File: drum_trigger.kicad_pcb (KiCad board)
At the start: 4 copper layers, 65 x 60 mm, 60 parts, among them J10 Conn_01x02_Pin, J11 Conn_01x02_Pin, J12 Conn_01x03_Pin, J4 Conn_01x03_Pin, J6 AudioJack2, J7 AudioJack2, U1 LM2902PWR

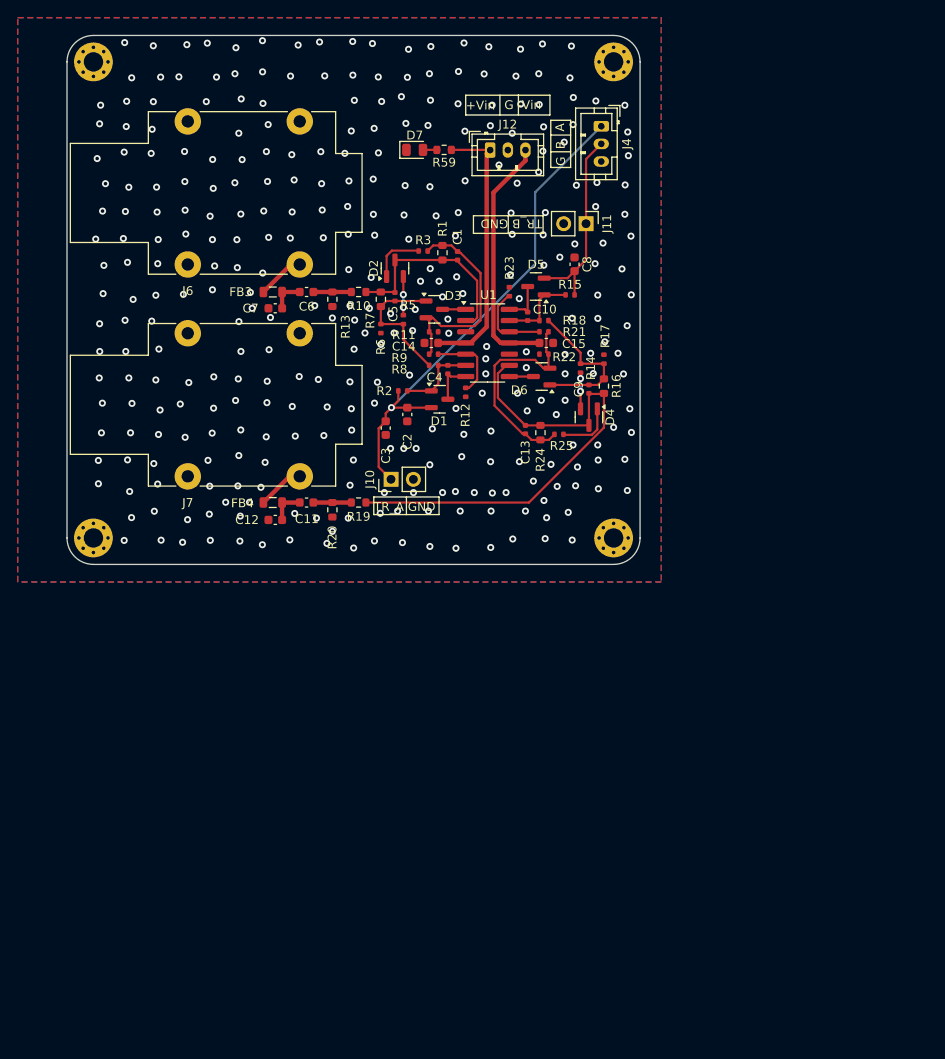
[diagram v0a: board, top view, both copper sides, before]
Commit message: Add channels
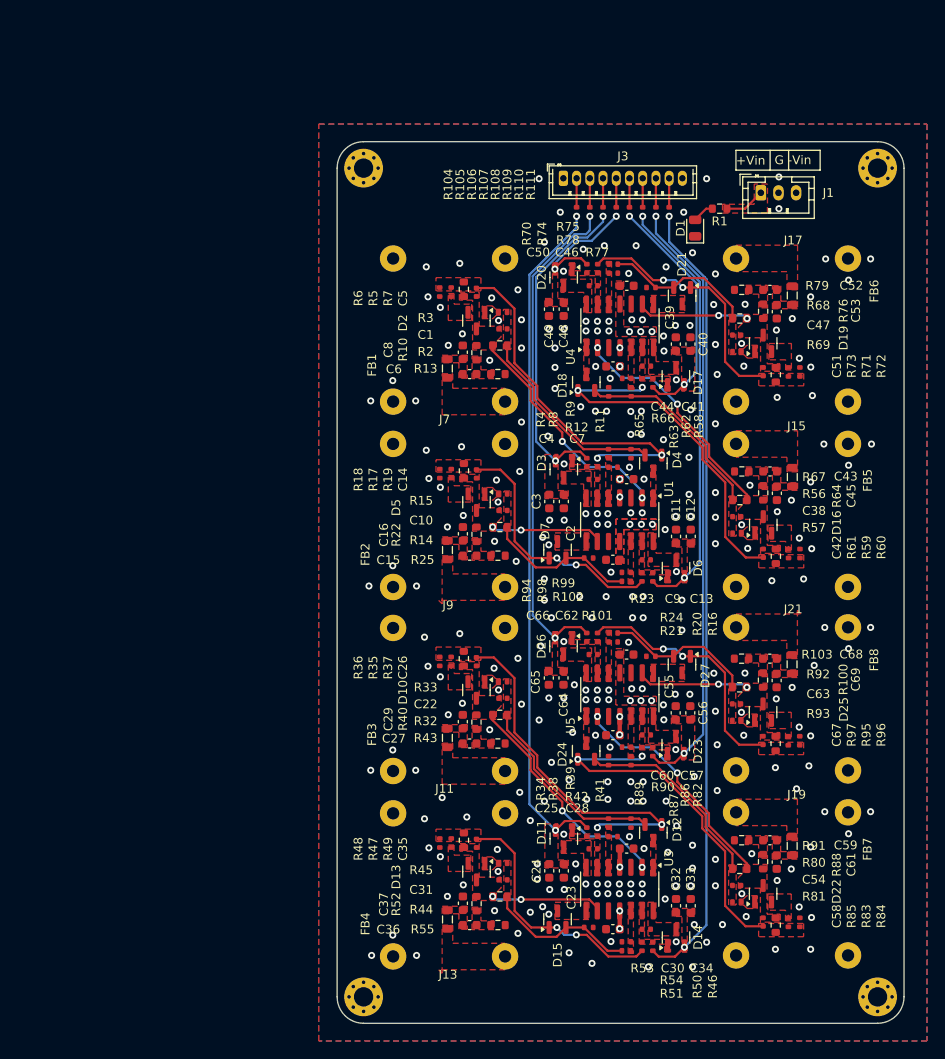
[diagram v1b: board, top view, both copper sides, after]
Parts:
- removed the D7 at (110.9, 42.9)
- removed J10: Conn_01x02_Pin, Connector_PinHeader_2.54mm:PinHeader_1x02_P2.54mm_Vertical
- removed J12, J4: Conn_01x03_Pin, Connector_JST:JST_PH_B3B-PH-K_1x03_P2.00mm_Vertical
- added C12: 1nF, Capacitor_SMD:C_0603_1608Metric, F.Cu at (142.2, 86.8)
- added C22: 22pF, C_0402_custom:C_0402_1005Metric, F.Cu at (120.9, 105.1)
- added C23: 220nF, Capacitor_SMD:C_0603_1608Metric, F.Cu at (127.8, 124.7)
- added C24: 1nF, Capacitor_SMD:C_0603_1608Metric, F.Cu at (126.2, 124.7)
- added C25: 22pF, C_0402_custom:C_0402_1005Metric, F.Cu at (131.1, 122.2)
- added C26: 22pF, C_0402_custom:C_0402_1005Metric, F.Cu at (117.9, 101.0)
- added C27: 220nF, Capacitor_SMD:C_0603_1608Metric, F.Cu at (117.1, 110.3)
- added C28: 1uF, Capacitor_SMD:C_0603_1608Metric, F.Cu at (134.9, 122.2)
- added C29: 100pF, Capacitor_SMD:C_0603_1608Metric, F.Cu at (116.4, 107.8)
- added C30: 1uF, Capacitor_SMD:C_0603_1608Metric, F.Cu at (133.4, 131.3)
- added C31: 22pF, C_0402_custom:C_0402_1005Metric, F.Cu at (120.9, 125.7)
- added C32: 220nF, Capacitor_SMD:C_0603_1608Metric, F.Cu at (140.5, 128.7)
- added C33: 1nF, Capacitor_SMD:C_0603_1608Metric, F.Cu at (142.2, 128.7)
- added C34: 22pF, C_0402_custom:C_0402_1005Metric, F.Cu at (137.2, 131.3)
- added C35: 22pF, C_0402_custom:C_0402_1005Metric, F.Cu at (117.9, 121.6)
- added C36: 220nF, Capacitor_SMD:C_0603_1608Metric, F.Cu at (117.1, 130.9)
- added C37: 100pF, Capacitor_SMD:C_0603_1608Metric, F.Cu at (116.4, 128.4)
- added C38: 22pF, C_0402_custom:C_0402_1005Metric, F.Cu at (147.4, 84.5)
- added C39: 220nF, Capacitor_SMD:C_0603_1608Metric, F.Cu at (140.5, 65.0)
- added C40: 1nF, Capacitor_SMD:C_0603_1608Metric, F.Cu at (142.2, 65.0)
- added C41: 22pF, C_0402_custom:C_0402_1005Metric, F.Cu at (137.2, 67.5)
- added C42: 22pF, C_0402_custom:C_0402_1005Metric, F.Cu at (150.4, 88.7)
- added C43: 220nF, Capacitor_SMD:C_0603_1608Metric, F.Cu at (151.2, 79.4)
- added C44: 1uF, Capacitor_SMD:C_0603_1608Metric, F.Cu at (133.4, 67.5)
- added C45: 100pF, Capacitor_SMD:C_0603_1608Metric, F.Cu at (152.0, 81.9)
- added C46: 1uF, Capacitor_SMD:C_0603_1608Metric, F.Cu at (135.0, 58.4)
- added C47: 22pF, C_0402_custom:C_0402_1005Metric, F.Cu at (147.4, 63.9)
- added C48: 220nF, Capacitor_SMD:C_0603_1608Metric, F.Cu at (127.8, 61.0)
- added C49: 1nF, Capacitor_SMD:C_0603_1608Metric, F.Cu at (126.1, 61.0)
- added C50: 22pF, C_0402_custom:C_0402_1005Metric, F.Cu at (131.2, 58.4)
- added C51: 22pF, C_0402_custom:C_0402_1005Metric, F.Cu at (150.4, 68.1)
- added C52: 220nF, Capacitor_SMD:C_0603_1608Metric, F.Cu at (151.2, 58.8)
- added C53: 100pF, Capacitor_SMD:C_0603_1608Metric, F.Cu at (152.0, 61.3)
- added C54: 22pF, C_0402_custom:C_0402_1005Metric, F.Cu at (147.4, 126.4)
- added C55: 220nF, Capacitor_SMD:C_0603_1608Metric, F.Cu at (140.5, 106.8)
- added C56: 1nF, Capacitor_SMD:C_0603_1608Metric, F.Cu at (142.2, 106.8)
- added C57: 22pF, C_0402_custom:C_0402_1005Metric, F.Cu at (137.2, 109.3)
- added C58: 22pF, C_0402_custom:C_0402_1005Metric, F.Cu at (150.4, 130.5)
- added C59: 220nF, Capacitor_SMD:C_0603_1608Metric, F.Cu at (151.2, 121.2)
- added C60: 1uF, Capacitor_SMD:C_0603_1608Metric, F.Cu at (133.4, 109.3)
- added C61: 100pF, Capacitor_SMD:C_0603_1608Metric, F.Cu at (152.0, 123.7)
- added C62: 1uF, Capacitor_SMD:C_0603_1608Metric, F.Cu at (134.9, 100.2)
- added C63: 22pF, C_0402_custom:C_0402_1005Metric, F.Cu at (147.4, 105.8)
- added C64: 220nF, Capacitor_SMD:C_0603_1608Metric, F.Cu at (127.8, 102.8)
- added C65: 1nF, Capacitor_SMD:C_0603_1608Metric, F.Cu at (126.1, 102.8)
- added C66: 22pF, C_0402_custom:C_0402_1005Metric, F.Cu at (131.1, 100.2)
- added C67: 22pF, C_0402_custom:C_0402_1005Metric, F.Cu at (150.4, 109.9)
- added C68: 220nF, Capacitor_SMD:C_0603_1608Metric, F.Cu at (151.2, 100.7)
- added C69: 100pF, Capacitor_SMD:C_0603_1608Metric, F.Cu at (152.0, 103.1)
- added D1: KT-0805G, LED_SMD:LED_0805_2012Metric, F.Cu at (142.7, 51.8)
- added D10: BAV99,215, Package_TO_SOT_SMD:SOT-23, F.Cu at (117.9, 104.2)
- added D11: BAV99,215, Package_TO_SOT_SMD:SOT-23, F.Cu at (127.8, 121.1)
- added D12: BAV99,215, Package_TO_SOT_SMD:SOT-23, F.Cu at (138.0, 120.4)
- added D13: BAV99,215, Package_TO_SOT_SMD:SOT-23, F.Cu at (117.9, 124.8)
- added D14: BAV99,215, Package_TO_SOT_SMD:SOT-23, F.Cu at (140.5, 132.3)
- added D15: BAV99,215, Package_TO_SOT_SMD:SOT-23, F.Cu at (127.1, 130.2)
- added D16: BAV99,215, Package_TO_SOT_SMD:SOT-23, F.Cu at (150.4, 85.5)
- added D17: BAV99,215, Package_TO_SOT_SMD:SOT-23, F.Cu at (140.5, 68.6)
- added D18: BAV99,215, Package_TO_SOT_SMD:SOT-23, F.Cu at (130.4, 69.3)
- added D19: BAV99,215, Package_TO_SOT_SMD:SOT-23, F.Cu at (150.4, 64.9)
- added D20: BAV99,215, Package_TO_SOT_SMD:SOT-23, F.Cu at (127.8, 57.4)
- added D21: BAV99,215, Package_TO_SOT_SMD:SOT-23, F.Cu at (141.2, 59.5)
- added D22: BAV99,215, Package_TO_SOT_SMD:SOT-23, F.Cu at (150.4, 127.3)
- added D23: BAV99,215, Package_TO_SOT_SMD:SOT-23, F.Cu at (140.5, 110.5)
- added D24: BAV99,215, Package_TO_SOT_SMD:SOT-23, F.Cu at (130.3, 111.1)
- added D25: BAV99,215, Package_TO_SOT_SMD:SOT-23, F.Cu at (150.4, 106.7)
- added D26: BAV99,215, Package_TO_SOT_SMD:SOT-23, F.Cu at (127.8, 99.2)
- added D27: BAV99,215, Package_TO_SOT_SMD:SOT-23, F.Cu at (141.2, 101.3)
- added FB3: 600, Inductor_SMD:L_0805_2012Metric, F.Cu at (114.6, 109.6)
- added FB4: 600, Inductor_SMD:L_0805_2012Metric, F.Cu at (114.6, 130.2)
- added FB5: 600, Inductor_SMD:L_0805_2012Metric, F.Cu at (153.7, 80.1)
- added FB6: 600, Inductor_SMD:L_0805_2012Metric, F.Cu at (153.7, 59.5)
- added FB7: 600, Inductor_SMD:L_0805_2012Metric, F.Cu at (153.7, 121.9)
- added FB8: 600, Inductor_SMD:L_0805_2012Metric, F.Cu at (153.7, 101.3)
- added J1: Conn_01x03_Pin, Connector_JST:JST_PH_B3B-PH-K_1x03_P2.00mm_Vertical, F.Cu at (150.2, 47.8)
- added J13: AudioJack2, Connector_Audio:Jack_6.35mm_Neutrik_NMJ4HFD2_Horizontal, F.Cu at (121.1, 134.4)
- added J15: AudioJack2, Connector_Audio:Jack_6.35mm_Neutrik_NMJ4HFD2_Horizontal, F.Cu at (147.3, 76.3)
- added J17: AudioJack2, Connector_Audio:Jack_6.35mm_Neutrik_NMJ4HFD2_Horizontal, F.Cu at (147.3, 55.3)
- added J19: AudioJack2, Connector_Audio:Jack_6.35mm_Neutrik_NMJ4HFD2_Horizontal, F.Cu at (147.3, 118.1)
- added J21: AudioJack2, Connector_Audio:Jack_6.35mm_Neutrik_NMJ4HFD2_Horizontal, F.Cu at (147.3, 97.1)
- added J3: Conn_01x10, Connector_JST:JST_ZH_B10B-ZR_1x10_P1.50mm_Vertical, F.Cu at (127.8, 46.2)
- added R1: 4.7k, Resistor_SMD:R_0603_1608Metric, F.Cu at (145.5, 49.6)
- added R100: 100k, Resistor_SMD:R_0603_1608Metric, F.Cu at (150.4, 103.1)
- added R101: 1k, R_0402_custom:R_0402_1005Metric, F.Cu at (137.7, 100.4)
- added R102: 22k, R_0402_custom:R_0402_1005Metric, F.Cu at (133.4, 98.8)
- added R103: 100k, Resistor_SMD:R_0603_1608Metric, F.Cu at (148.0, 100.7)
- added R104: 100, R_0402_custom:R_0402_1005Metric, F.Cu at (129.3, 50.0)
- added R105: 100, R_0402_custom:R_0402_1005Metric, F.Cu at (130.8, 50.0)
- added R106: 100, R_0402_custom:R_0402_1005Metric, F.Cu at (132.3, 50.0)
- added R107: 100, R_0402_custom:R_0402_1005Metric, F.Cu at (133.8, 50.0)
- added R108: 100, R_0402_custom:R_0402_1005Metric, F.Cu at (135.3, 50.0)
- added R109: 100, R_0402_custom:R_0402_1005Metric, F.Cu at (136.8, 50.0)
- added R110: 100, R_0402_custom:R_0402_1005Metric, F.Cu at (138.3, 50.0)
- added R111: 100, R_0402_custom:R_0402_1005Metric, F.Cu at (139.8, 50.0)
- added R32: 68k, Resistor_SMD:R_0603_1608Metric, F.Cu at (120.6, 107.0)
- added R33: 10k, R_0402_custom:R_0402_1005Metric, F.Cu at (120.9, 103.3)
- added R34: 22k, R_0402_custom:R_0402_1005Metric, F.Cu at (130.4, 120.3)
- added R35: 10k, R_0402_custom:R_0402_1005Metric, F.Cu at (115.0, 101.0)
- added R36: 1k, R_0402_custom:R_0402_1005Metric, F.Cu at (113.7, 101.0)
- added R37: 68k, Resistor_SMD:R_0603_1608Metric, F.Cu at (116.5, 100.6)
- added R38: 22k, R_0402_custom:R_0402_1005Metric, F.Cu at (131.6, 120.3)
- added R39: 22k, R_0402_custom:R_0402_1005Metric, F.Cu at (132.9, 119.3)
- added R40: 100k, Resistor_SMD:R_0603_1608Metric, F.Cu at (117.9, 107.8)
- added R41: 1k, R_0402_custom:R_0402_1005Metric, F.Cu at (135.4, 119.3)
- added R42: 22k, R_0402_custom:R_0402_1005Metric, F.Cu at (133.4, 120.8)
- added R43: 100k, Resistor_SMD:R_0603_1608Metric, F.Cu at (120.3, 110.3)
- added R44: 68k, Resistor_SMD:R_0603_1608Metric, F.Cu at (120.6, 127.6)
- added R45: 10k, R_0402_custom:R_0402_1005Metric, F.Cu at (120.9, 123.9)
- added R46: 22k, R_0402_custom:R_0402_1005Metric, F.Cu at (137.9, 133.3)
- added R47: 10k, R_0402_custom:R_0402_1005Metric, F.Cu at (115.0, 121.6)
- added R48: 1k, R_0402_custom:R_0402_1005Metric, F.Cu at (113.7, 121.6)
- added R49: 68k, Resistor_SMD:R_0603_1608Metric, F.Cu at (116.5, 121.2)
- added R50: 22k, R_0402_custom:R_0402_1005Metric, F.Cu at (136.7, 133.3)
- added R51: 22k, R_0402_custom:R_0402_1005Metric, F.Cu at (134.9, 133.8)
- added R52: 100k, Resistor_SMD:R_0603_1608Metric, F.Cu at (117.9, 128.4)
- added R53: 1k, R_0402_custom:R_0402_1005Metric, F.Cu at (130.6, 131.1)
- added R54: 22k, R_0402_custom:R_0402_1005Metric, F.Cu at (134.9, 132.8)
- added R55: 100k, Resistor_SMD:R_0603_1608Metric, F.Cu at (120.3, 130.9)
- added R56: 68k, Resistor_SMD:R_0603_1608Metric, F.Cu at (147.8, 82.7)
- added R57: 10k, R_0402_custom:R_0402_1005Metric, F.Cu at (147.5, 86.4)
- added R58: 22k, R_0402_custom:R_0402_1005Metric, F.Cu at (137.9, 69.4)
- added R60: 1k, R_0402_custom:R_0402_1005Metric, F.Cu at (154.6, 88.7)
- added R61: 68k, Resistor_SMD:R_0603_1608Metric, F.Cu at (151.9, 89.0)
- added R62: 22k, R_0402_custom:R_0402_1005Metric, F.Cu at (136.7, 69.4)
- added R63: 22k, R_0402_custom:R_0402_1005Metric, F.Cu at (135.5, 70.4)
- added R64: 100k, Resistor_SMD:R_0603_1608Metric, F.Cu at (150.4, 81.8)
- added R65: 1k, R_0402_custom:R_0402_1005Metric, F.Cu at (132.9, 70.4)
- added R66: 22k, R_0402_custom:R_0402_1005Metric, F.Cu at (134.9, 68.9)
- added R67: 100k, Resistor_SMD:R_0603_1608Metric, F.Cu at (148.0, 79.4)
- added R68: 68k, Resistor_SMD:R_0603_1608Metric, F.Cu at (147.8, 62.1)
- added R69: 10k, R_0402_custom:R_0402_1005Metric, F.Cu at (147.5, 65.8)
- added R70: 22k, R_0402_custom:R_0402_1005Metric, F.Cu at (130.4, 56.4)
- added R71: 10k, R_0402_custom:R_0402_1005Metric, F.Cu at (153.3, 68.1)
- added R72: 1k, R_0402_custom:R_0402_1005Metric, F.Cu at (154.6, 68.1)
- added R73: 68k, Resistor_SMD:R_0603_1608Metric, F.Cu at (151.9, 68.4)
- added R74: 22k, R_0402_custom:R_0402_1005Metric, F.Cu at (131.7, 56.4)
- added R75: 22k, R_0402_custom:R_0402_1005Metric, F.Cu at (133.4, 55.9)
- added R76: 100k, Resistor_SMD:R_0603_1608Metric, F.Cu at (150.4, 61.2)
- added R77: 1k, R_0402_custom:R_0402_1005Metric, F.Cu at (137.7, 58.6)
- added R78: 22k, R_0402_custom:R_0402_1005Metric, F.Cu at (133.4, 56.9)
- added R79: 100k, Resistor_SMD:R_0603_1608Metric, F.Cu at (148.0, 58.8)
- added R80: 68k, Resistor_SMD:R_0603_1608Metric, F.Cu at (147.8, 124.5)
- added R81: 10k, R_0402_custom:R_0402_1005Metric, F.Cu at (147.4, 128.3)
- added R82: 22k, R_0402_custom:R_0402_1005Metric, F.Cu at (137.9, 111.2)
- added R83: 10k, R_0402_custom:R_0402_1005Metric, F.Cu at (153.3, 130.6)
- added R84: 1k, R_0402_custom:R_0402_1005Metric, F.Cu at (154.6, 130.6)
- added R85: 68k, Resistor_SMD:R_0603_1608Metric, F.Cu at (151.8, 130.9)
- added R86: 22k, R_0402_custom:R_0402_1005Metric, F.Cu at (136.7, 111.2)
- added R87: 22k, R_0402_custom:R_0402_1005Metric, F.Cu at (135.4, 112.2)
- added R88: 100k, Resistor_SMD:R_0603_1608Metric, F.Cu at (150.4, 123.7)
- added R89: 1k, R_0402_custom:R_0402_1005Metric, F.Cu at (132.9, 112.2)
- added R90: 22k, R_0402_custom:R_0402_1005Metric, F.Cu at (134.9, 110.7)
- added R91: 100k, Resistor_SMD:R_0603_1608Metric, F.Cu at (148.0, 121.2)
- added R92: 68k, Resistor_SMD:R_0603_1608Metric, F.Cu at (147.8, 103.9)
- added R93: 10k, R_0402_custom:R_0402_1005Metric, F.Cu at (147.4, 107.7)
- added R94: 22k, R_0402_custom:R_0402_1005Metric, F.Cu at (130.4, 98.2)
- added R95: 10k, R_0402_custom:R_0402_1005Metric, F.Cu at (153.3, 110.0)
- added R96: 1k, R_0402_custom:R_0402_1005Metric, F.Cu at (154.6, 110.0)
- added R97: 68k, Resistor_SMD:R_0603_1608Metric, F.Cu at (151.8, 110.3)
- added R98: 22k, R_0402_custom:R_0402_1005Metric, F.Cu at (131.6, 98.2)
- added R99: 22k, R_0402_custom:R_0402_1005Metric, F.Cu at (133.4, 97.7)
- added U3: LM324DT, Package_SO:SOIC-14_3.9x8.7mm_P1.27mm, F.Cu at (134.1, 126.8)
- added U4: LM324DT, Package_SO:SOIC-14_3.9x8.7mm_P1.27mm, F.Cu at (134.2, 62.9)
- added U5: LM324DT, Package_SO:SOIC-14_3.9x8.7mm_P1.27mm, F.Cu at (134.2, 104.7)
- J11: value Conn_01x02_Pin -> AudioJack2; footprint Connector_PinHeader_2.54mm:PinHeader_1x02_P2.54mm_Vertical -> Connector_Audio:Jack_6.35mm_Neutrik_NMJ4HFD2_Horizontal
- R59: value 1.5k -> 10k; footprint Resistor_SMD:R_0603_1608Metric -> R_0402_custom:R_0402_1005Metric
- U1: value LM2902PWR -> LM324DT
- moved H4 103.1 mm to (163.4, 139.0)
- moved J11 62.8 mm to (121.1, 113.4), turned to 180 degrees
- moved R59 60.2 mm to (153.3, 88.7), turned to -90 degrees
- moved H3 59.3 mm to (105.1, 139.0)
- moved D6 35.7 mm to (140.5, 90.4), turned to 90 degrees
- moved R24 34.5 mm to (134.9, 90.9), turned to 0 degrees
- moved R16 33.3 mm to (137.9, 91.4), turned to -90 degrees
- moved C11 32.9 mm to (140.5, 86.8)
- moved H1 32.9 mm to (105.1, 45.0)
- moved H2 32.3 mm to (163.4, 45.0)
- moved R20 31.1 mm to (136.7, 91.4), turned to 90 degrees
- moved C13 30.7 mm to (137.2, 89.4), turned to 0 degrees
- moved D4 30.4 mm to (138.0, 78.5), turned to -90 degrees
- moved R21 29.8 mm to (134.9, 91.9), turned to 0 degrees
- moved J7 28.0 mm to (121.1, 71.5)
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- renumbered C9 to C10, C8 to C11, C10 to C13, C13 to C14, C11 to C15, C12 to C16, C14 to C7, C7 to C8, C15 to C9, D1 to D3, D3 to D4, D4 to D5, D5 to D6, D6 to D7, FB3 to FB1, FB4 to FB2, J6 to J7, J7 to J9, R16 to R14, R14 to R15, R15 to R16, R25 to R17, R17 to R18, R24 to R19, R1 to R2, R18 to R20, R19 to R22, R22 to R23, R23 to R24, R20 to R25, R2 to R4
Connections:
- net /TriggerPair/TRIG_A_IN renamed TRIG1_IN
- net /TriggerPair/TRIG_A_OUT renamed TRIG_T1
- net /TriggerPair/TRIG_B_IN renamed TRIG2_IN
- C10 pad 2: Net-(C9-Pad2) -> Net-(D7-A)
- C11 pad 2: /TriggerPair/TRIG_B_OUT -> TRIG_T2
- C14 pad 1: Net-(U1C--) -> Net-(C14-Pad1)
- C14 pad 2: Net-(D6-A) -> Net-(U1C--)
- D5 pad 1: Net-(D4-K-Pad1) -> Net-(D5-K-Pad1)
- D5 pad 2: Net-(D4-A) (its old number) -> Net-(D5-A)
- D6 pad 2: /TriggerPair/TRIG_B_OUT -> TRIG_T2
- D7 pad 1: Net-(C9-Pad2) -> Net-(C14-Pad1)
- D7 pad 2: Net-(D6-A) -> Net-(D7-A)
- R14 pad 1: Net-(C9-Pad2) -> Net-(D7-A)
- R15 pad 1: Net-(C9-Pad2) -> Net-(D7-A)
- R15 pad 2: Net-(D4-A) (its old number) -> Net-(D5-K-Pad1)
- R16 pad 2: /TriggerPair/TRIG_B_OUT -> TRIG_T2
- R17 pad 1: Net-(D6-A) -> Net-(D5-A)
- R17 pad 2: Net-(D4-K-Pad1) -> Net-(C14-Pad1)
- R18 pad 2: Net-(C9-Pad2) -> Net-(C14-Pad1)
- R19 pad 1: Net-(D6-A) -> Net-(C14-Pad1)
- R20 pad 1: Net-(C9-Pad2) -> Net-(C14-Pad1)
- R21 pad 1: Net-(D6-A) -> Net-(D7-A)
- R23 pad 1: Net-(D6-A) -> Net-(D7-A)
- R59 pad 1: +9V -> Net-(D16-A)
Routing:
- net TRIG_T4: track 0.00 -> 90.0 mm, vias 0 -> 2
- net TRIG_T3: track 0.00 -> 77.4 mm, vias 0 -> 2
- net TRIG_T7: track 0.00 -> 68.3 mm, vias 0 -> 2
- net TRIG_T8: track 0.00 -> 56.6 mm, vias 0 -> 2
- net TRIG_T2: track 0.00 -> 48.6 mm, vias 0 -> 2
- net Net-(U1C--): track 55.8 -> 12.4 mm, vias 0 -> 2
- net Net-(C26-Pad2): track 0.00 -> 40.8 mm, vias 0 -> 2
- net Net-(C58-Pad2): track 0.00 -> 40.8 mm, vias 0 -> 2
- net Net-(C42-Pad2): track 1.89 -> 40.8 mm, vias 0 -> 2
- net Net-(C35-Pad1): track 0.00 -> 28.4 mm, vias 0 -> 2
- net Net-(C67-Pad1): track 0.00 -> 28.4 mm, vias 0 -> 2
- net Net-(C51-Pad1): track 0.00 -> 28.4 mm, vias 0 -> 2
- net Net-(C14-Pad1): track 0.00 -> 28.4 mm, vias 0 -> 2
- net TRIG_T5: track 0.00 -> 27.1 mm, vias 0 -> 2
- net Net-(U3A--): track 0.00 -> 26.3 mm, vias 0 -> 2
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- added copper zone on F.Cu, net +9V
- added copper zone on In1.Cu, net +9V
- added copper zone on F.Cu, net -9V
- added copper zone on In2.Cu, net -9V
- added copper zone on F.Cu, net Net-(C13-Pad2)
- added copper zone on F.Cu, net Net-(C14-Pad1)
- added copper zone on F.Cu, net Net-(C15-Pad1)
- added copper zone on F.Cu, net Net-(C15-Pad2)
- added copper zone on F.Cu, net Net-(C25-Pad2)
- added copper zone on F.Cu, net Net-(C26-Pad2)
- added copper zone on F.Cu, net Net-(C27-Pad1)
- added copper zone on F.Cu, net Net-(C27-Pad2)
- added copper zone on F.Cu, net Net-(C34-Pad2)
- added copper zone on F.Cu, net Net-(C35-Pad1)
- added copper zone on F.Cu, net Net-(C36-Pad1)
- added copper zone on F.Cu, net Net-(C36-Pad2)
- added copper zone on F.Cu, net Net-(C4-Pad2)
- added copper zone on F.Cu, net Net-(C41-Pad2)
- added copper zone on F.Cu, net Net-(C42-Pad2)
- added copper zone on F.Cu, net Net-(C43-Pad1)
- added copper zone on F.Cu, net Net-(C43-Pad2)
- added copper zone on F.Cu, net Net-(C5-Pad2)
- added copper zone on F.Cu, net Net-(C50-Pad2)
- added copper zone on F.Cu, net Net-(C51-Pad1)
- added copper zone on F.Cu, net Net-(C52-Pad1)
- added copper zone on F.Cu, net Net-(C52-Pad2)
- added copper zone on F.Cu, net Net-(C57-Pad2)
- added copper zone on F.Cu, net Net-(C58-Pad2)
- added copper zone on F.Cu, net Net-(C59-Pad1)
- added copper zone on F.Cu, net Net-(C59-Pad2)
- added copper zone on F.Cu, net Net-(C6-Pad1)
- added copper zone on F.Cu, net Net-(C6-Pad2)
- added copper zone on F.Cu, net Net-(C66-Pad2)
- added copper zone on F.Cu, net Net-(C67-Pad1)
- added copper zone on F.Cu, net Net-(C68-Pad1)
- added copper zone on F.Cu, net Net-(C68-Pad2)
- added copper zone on F.Cu, net Net-(D10-A)
- added copper zone on F.Cu, net Net-(D10-K-Pad1)
- added copper zone on F.Cu, net Net-(D12-A)
- added copper zone on F.Cu, net Net-(D12-K-Pad3)
- added copper zone on F.Cu, net Net-(D13-A)
- added copper zone on F.Cu, net Net-(D13-K-Pad1)
- added copper zone on F.Cu, net Net-(D15-A)
- added copper zone on F.Cu, net Net-(D15-K-Pad3)
- added copper zone on F.Cu, net Net-(D16-A)
- added copper zone on F.Cu, net Net-(D16-K-Pad1)
- added copper zone on F.Cu, net Net-(D18-A)
- added copper zone on F.Cu, net Net-(D18-K-Pad3)
- added copper zone on F.Cu, net Net-(D19-A)
- added copper zone on F.Cu, net Net-(D19-K-Pad1)
- added copper zone on F.Cu, net Net-(D2-A)
- added copper zone on F.Cu, net Net-(D2-K-Pad1)
- added copper zone on F.Cu, net Net-(D21-A)
- added copper zone on F.Cu, net Net-(D21-K-Pad3)
- added copper zone on F.Cu, net Net-(D22-A)
- added copper zone on F.Cu, net Net-(D22-K-Pad1)
- added copper zone on F.Cu, net Net-(D24-A)
- added copper zone on F.Cu, net Net-(D24-K-Pad3)
- added copper zone on F.Cu, net Net-(D25-A)
- added copper zone on F.Cu, net Net-(D25-K-Pad1)
- added copper zone on F.Cu, net Net-(D27-A)
- added copper zone on F.Cu, net Net-(D27-K-Pad3)
- added copper zone on F.Cu, net Net-(D4-A)
- added copper zone on F.Cu, net Net-(D4-K-Pad3)
- added copper zone on F.Cu, net Net-(D5-A)
- added copper zone on F.Cu, net Net-(D5-K-Pad1)
- added copper zone on F.Cu, net Net-(D7-A)
- added copper zone on F.Cu, net Net-(D7-K-Pad3)
- added copper zone on F.Cu, net Net-(U1A--)
- added copper zone on F.Cu, net Net-(U1B-+)
- added copper zone on F.Cu, net Net-(U1B--)
- added copper zone on F.Cu, net Net-(U1C--)
- added copper zone on F.Cu, net Net-(U1D-+)
- added copper zone on F.Cu, net Net-(U1D--)
- added copper zone on F.Cu, net Net-(U3A--)
- added copper zone on F.Cu, net Net-(U3B-+)
- added copper zone on F.Cu, net Net-(U3B--)
- added copper zone on F.Cu, net Net-(U3C--)
- added copper zone on F.Cu, net Net-(U3D-+)
- added copper zone on F.Cu, net Net-(U3D--)
- added copper zone on F.Cu, net Net-(U4A--)
- added copper zone on F.Cu, net Net-(U4B-+)
- added copper zone on F.Cu, net Net-(U4B--)
- added copper zone on F.Cu, net Net-(U4C--)
- added copper zone on F.Cu, net Net-(U4D-+)
- added copper zone on F.Cu, net Net-(U4D--)
- added copper zone on F.Cu, net Net-(U5A--)
- added copper zone on F.Cu, net Net-(U5B-+)
- added copper zone on F.Cu, net Net-(U5B--)
- added copper zone on F.Cu, net Net-(U5C--)
- added copper zone on F.Cu, net Net-(U5D-+)
- added copper zone on F.Cu, net Net-(U5D--)
- added copper zone on F.Cu, net TRIG1_IN
- added copper zone on F.Cu, net TRIG2_IN
- added copper zone on F.Cu, net TRIG3_IN
- added copper zone on F.Cu, net TRIG4_IN
- added copper zone on F.Cu, net TRIG5_IN
- added copper zone on F.Cu, net TRIG6_IN
- added copper zone on F.Cu, net TRIG7_IN
- added copper zone on F.Cu, net TRIG8_IN
- added copper zone on F.Cu, net TRIG_T1
- added copper zone on F.Cu, net TRIG_T2
- added copper zone on F.Cu, net TRIG_T3
- added copper zone on F.Cu, net TRIG_T4
- added copper zone on F.Cu, net TRIG_T5
- added copper zone on F.Cu, net TRIG_T6
- added copper zone on F.Cu, net TRIG_T7
- added copper zone on F.Cu, net TRIG_T8
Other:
- board size 65 x 60 mm -> 64.3 x 100 mm
- board text removed: "A"
- board text removed: "B"
- board text removed: "TR_A GND"
- board text removed: "TR_B GND"
